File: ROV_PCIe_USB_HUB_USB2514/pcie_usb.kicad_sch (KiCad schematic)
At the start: 37 parts, among them U1 UPD720201K8-701-BAC-A, U2 SST25VF512A-33-4C-SAE, Y1 ABM8-24.000MHZ-B2-T

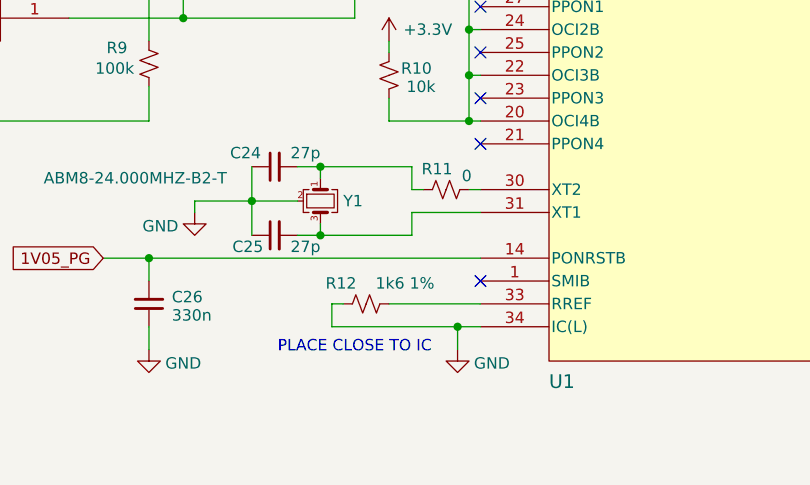
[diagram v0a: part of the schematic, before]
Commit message: updates
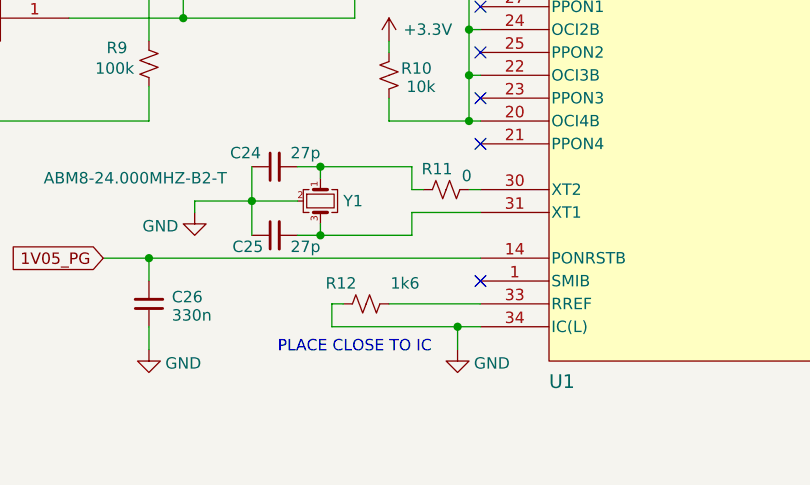
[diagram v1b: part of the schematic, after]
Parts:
- C10: Part Number CL21A106KOQNNNE -> CL21A106KOQNNNE
- C11, C12, C13, C14, C15, C16, C17, C18, C19, C20, C22, C23, C3, C4, C5, C6, C7, C8: Part Number CL05B104KB5NNNC -> CL05B104KO5NNNC
- C21, C9: footprint Capacitor_SMD:C_1206_3216Metric -> Capacitor_SMD:C_0805_2012Metric; Part Number CL31B226MPHNNNE -> CL21A226MOQNNNE
- C24, C25: Part Number CL05C270JB51PNC -> CL05C270JB5NNNC
- R10, R4, R5, R6, R7, R8: Part Number AC0603FR-0710KL -> RC0603FR-0710KL
- R11: Part Number AC0402FR-070RL -> RC0402JR-070RL
- R12: value 1k6 1% -> 1k6; Part Number RT0603BRD071K6L -> RC0603FR-071K6L
- R9: Part Number AC0603FR-07100KL -> RC0603FR-07100KL
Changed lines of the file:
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@@
 			)
 		)
-		(property "Part Number" "AC0603FR-0710KL"
+		(property "Part Number" "RC0603FR-0710KL"
 			(at 107.95 116.84 0)
 			(hide yes)
@@
 			)
 		)
-		(property "Part Number" "CL05B104KB5NNNC"
+		(property "Part Number" "CL05B104KO5NNNC"
 			(at 29.21 29.21 0)
 			(hide yes)
@@
 			)
 		)
-		(property "Part Number" "AC0603FR-07100KL"
+		(property "Part Number" "RC0603FR-07100KL"
 			(at 81.28 115.57 0)
 			(hide yes)
@@
 			)
 		)
-		(property "Part Number" "CL05B104KB5NNNC"
+		(property "Part Number" "CL05B104KO5NNNC"
 			(at 39.37 46.99 0)
 			(hide yes)
@@
 			)
 		)
-		(property "Part Number" "CL05B104KB5NNNC"
+		(property "Part Number" "CL05B104KO5NNNC"
 			(at 91.44 59.69 90)
 			(hide yes)
@@
 			)
 		)
-		(property "Part Number" "AC0402FR-070RL"
+		(property "Part Number" "RC0402JR-070RL"
 			(at 114.3 129.54 90)
 			(hide yes)
@@
 			)
 		)
-		(property "Part Number" "AC0603FR-0710KL"
+		(property "Part Number" "RC0603FR-0710KL"
 			(at 85.09 96.52 0)
 			(hide yes)
@@
 			)
 		)
-		(property "Part Number" "CL05C270JB51PNC"
+		(property "Part Number" "CL05C270JB5NNNC"
 			(at 95.25 127 90)
 			(hide yes)
@@
 			)
 		)
-		(property "Part Number" "CL05B104KB5NNNC"
+		(property "Part Number" "CL05B104KO5NNNC"
 			(at 34.29 29.21 0)
 			(hide yes)
@@
 			)
 		)
-		(property "Part Number" "CL05B104KB5NNNC"
+		(property "Part Number" "CL05B104KO5NNNC"
 			(at 64.77 46.99 0)
 			(hide yes)
@@
 			)
 		)
-		(property "Footprint" "Capacitor_SMD:C_1206_3216Metric"
+		(property "Footprint" "Capacitor_SMD:C_0805_2012Metric"
 			(at 64.77 29.21 0)
 			(hide yes)
@@
 			)
 		)
-		(property "Part Number" "CL31B226MPHNNNE"
+		(property "Part Number" "CL21A226MOQNNNE"
 			(at 64.77 29.21 0)
 			(hide yes)
@@
 			)
 		)
-		(property "Part Number" "CL05B104KB5NNNC"
+		(property "Part Number" "CL05B104KO5NNNC"
 			(at 49.53 29.21 0)
 			(hide yes)
@@
 			)
 		)
-		(property "Part Number" "CL05B104KB5NNNC"
+		(property "Part Number" "CL05B104KO5NNNC"
 			(at 34.29 46.99 0)
 			(hide yes)
@@
 			)
 		)
-		(property "Part Number" "CL05C270JB51PNC"
+		(property "Part Number" "CL05C270JB5NNNC"
 			(at 95.25 134.62 90)
 			(hide yes)
@@
 			)
 		)
-		(property "Part Number" "CL05B104KB5NNNC"
+		(property "Part Number" "CL05B104KO5NNNC"
 			(at 223.52 39.37 0)
 			(hide yes)
@@
 			)
 		)
-		(property "Part Number" "AC0603FR-0710KL"
+		(property "Part Number" "RC0603FR-0710KL"
 			(at 77.47 96.52 0)
 			(hide yes)
@@
 			)
 		)
-		(property "Footprint" "Capacitor_SMD:C_1206_3216Metric"
+		(property "Footprint" "Capacitor_SMD:C_0805_2012Metric"
 			(at 73.66 46.99 0)
 			(hide yes)
@@
 			)
 		)
-		(property "Part Number" "CL31B226MPHNNNE"
+		(property "Part Number" "CL21A226MOQNNNE"
 			(at 73.66 46.99 0)
 			(hide yes)
@@
 			)
 		)
-		(property "Part Number" "CL05B104KB5NNNC"
+		(property "Part Number" "CL05B104KO5NNNC"
 			(at 59.69 46.99 0)
 			(hide yes)
@@
 			)
 		)
-		(property "Part Number" "CL05B104KB5NNNC"
+		(property "Part Number" "CL05B104KO5NNNC"
 			(at 49.53 46.99 0)
 			(hide yes)
@@
 			)
 		)
-		(property "Part Number" "AC0603FR-0710KL"
+		(property "Part Number" "RC0603FR-0710KL"
 			(at 73.66 96.52 0)
 			(hide yes)
@@
 			)
 		)
-		(property "Part Number" "CL05B104KB5NNNC"
+		(property "Part Number" "CL05B104KO5NNNC"
 			(at 44.45 46.99 0)
 			(hide yes)
@@
 			)
 		)
-		(property "Part Number" "CL05B104KB5NNNC"
+		(property "Part Number" "CL05B104KO5NNNC"
 			(at 91.44 62.23 90)
 			(hide yes)
@@
 			)
 		)
-		(property "Part Number" "CL21A106KOQNNNE"
+		(property "Part Number" "CL21A106KOQNNNE "
 			(at 213.36 39.37 0)
 			(hide yes)
@@
 			)
 		)
-		(property "Part Number" "CL05B104KB5NNNC"
+		(property "Part Number" "CL05B104KO5NNNC"
 			(at 39.37 29.21 0)
 			(hide yes)
@@
 			)
 		)
-		(property "Part Number" "CL05B104KB5NNNC"
+		(property "Part Number" "CL05B104KO5NNNC"
 			(at 44.45 29.21 0)
 			(hide yes)
@@
 			)
 		)
-		(property "Value" "1k6 1%"
+		(property "Value" "1k6"
 			(at 109.728 139.954 90)
 			(show_name no)
@@
 			)
 		)
-		(property "Part Number" "RT0603BRD071K6L"
+		(property "Part Number" "RC0603FR-071K6L"
 			(at 105.41 142.24 90)
 			(hide yes)
@@
 			)
 		)
-		(property "Part Number" "CL05B104KB5NNNC"
+		(property "Part Number" "CL05B104KO5NNNC"
 			(at 54.61 46.99 0)
 			(hide yes)
@@
 			)
 		)
-		(property "Part Number" "CL05B104KB5NNNC"
+		(property "Part Number" "CL05B104KO5NNNC"
 			(at 54.61 29.21 0)
 			(hide yes)
@@
 			)
 		)
-		(property "Part Number" "CL05B104KB5NNNC"
+		(property "Part Number" "CL05B104KO5NNNC"
 			(at 228.6 39.37 0)
 			(hide yes)
@@
 			)
 		)
-		(property "Part Number" "AC0603FR-0710KL"
+		(property "Part Number" "RC0603FR-0710KL"
 			(at 81.28 77.47 0)
 			(hide yes)
@@
 			)
 		)
-		(property "Part Number" "AC0603FR-0710KL"
+		(property "Part Number" "RC0603FR-0710KL"
 			(at 38.1 101.6 0)
 			(hide yes)
@@
 			)
 		)
-		(property "Part Number" "CL05B104KB5NNNC"
+		(property "Part Number" "CL05B104KO5NNNC"
 			(at 29.21 46.99 0)
 			(hide yes)

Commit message: changes
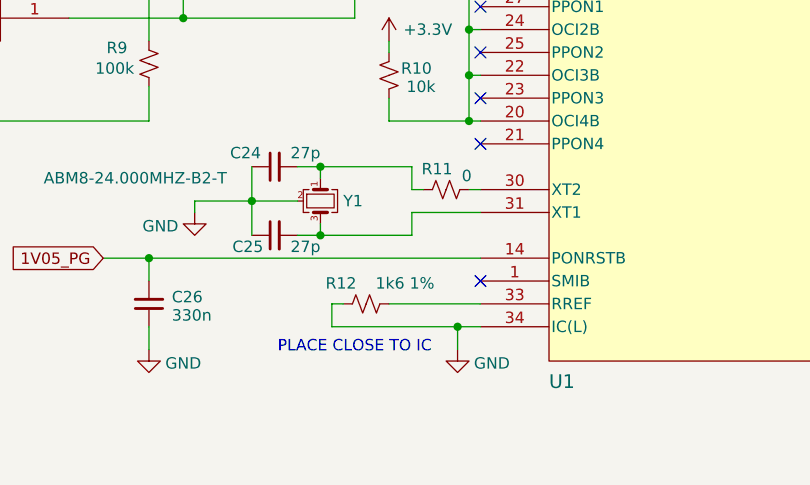
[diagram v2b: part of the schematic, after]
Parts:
- C10: Part Number CL21A106KOQNNNE -> CC0805KRX5R8BB106
- C11, C12, C13, C14, C15, C16, C17, C18, C19, C20, C22, C23, C3, C4, C5, C6, C7, C8: Part Number CL05B104KO5NNNC -> CC0402KRX7R8BB104
- C21, C9: footprint Capacitor_SMD:C_0805_2012Metric -> Capacitor_SMD:C_1206_3216Metric; Part Number CL21A226MOQNNNE -> CC1206KKX5R8BB226
- C24, C25: Part Number CL05C270JB5NNNC -> CC0402JRNPO9BN270
- C26: Part Number CL05A334KQ5NNNC -> CC0402KPX5R6BB334
- R12: value 1k6 -> 1k6 1%
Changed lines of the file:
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@@
 			)
 		)
-		(property "Part Number" "CL05B104KO5NNNC"
+		(property "Part Number" "CC0402KRX7R8BB104"
 			(at 29.21 29.21 0)
 			(hide yes)
@@
 			)
 		)
-		(property "Part Number" "CL05B104KO5NNNC"
+		(property "Part Number" "CC0402KRX7R8BB104"
 			(at 39.37 46.99 0)
 			(hide yes)
@@
 			)
 		)
-		(property "Part Number" "CL05B104KO5NNNC"
+		(property "Part Number" "CC0402KRX7R8BB104"
 			(at 91.44 59.69 90)
 			(hide yes)
@@
 			)
 		)
-		(property "Part Number" "CL05C270JB5NNNC"
+		(property "Part Number" "CC0402JRNPO9BN270"
 			(at 95.25 127 90)
 			(hide yes)
@@
 			)
 		)
-		(property "Part Number" "CL05B104KO5NNNC"
+		(property "Part Number" "CC0402KRX7R8BB104"
 			(at 34.29 29.21 0)
 			(hide yes)
@@
 			)
 		)
-		(property "Part Number" "CL05B104KO5NNNC"
+		(property "Part Number" "CC0402KRX7R8BB104"
 			(at 64.77 46.99 0)
 			(hide yes)
@@
 			)
 		)
-		(property "Footprint" "Capacitor_SMD:C_0805_2012Metric"
+		(property "Footprint" "Capacitor_SMD:C_1206_3216Metric"
 			(at 64.77 29.21 0)
 			(hide yes)
@@
 			)
 		)
-		(property "Part Number" "CL21A226MOQNNNE"
+		(property "Part Number" "CC1206KKX5R8BB226"
 			(at 64.77 29.21 0)
 			(hide yes)
@@
 			)
 		)
-		(property "Part Number" "CL05B104KO5NNNC"
+		(property "Part Number" "CC0402KRX7R8BB104"
 			(at 49.53 29.21 0)
 			(hide yes)
@@
 			)
 		)
-		(property "Part Number" "CL05B104KO5NNNC"
+		(property "Part Number" "CC0402KRX7R8BB104"
 			(at 34.29 46.99 0)
 			(hide yes)
@@
 			)
 		)
-		(property "Part Number" "CL05C270JB5NNNC"
+		(property "Part Number" "CC0402JRNPO9BN270"
 			(at 95.25 134.62 90)
 			(hide yes)
@@
 			)
 		)
-		(property "Part Number" "CL05B104KO5NNNC"
+		(property "Part Number" "CC0402KRX7R8BB104"
 			(at 223.52 39.37 0)
 			(hide yes)
@@
 			)
 		)
-		(property "Footprint" "Capacitor_SMD:C_0805_2012Metric"
+		(property "Footprint" "Capacitor_SMD:C_1206_3216Metric"
 			(at 73.66 46.99 0)
 			(hide yes)
@@
 			)
 		)
-		(property "Part Number" "CL21A226MOQNNNE"
+		(property "Part Number" "CC1206KKX5R8BB226"
 			(at 73.66 46.99 0)
 			(hide yes)
@@
 			)
 		)
-		(property "Part Number" "CL05B104KO5NNNC"
+		(property "Part Number" "CC0402KRX7R8BB104"
 			(at 59.69 46.99 0)
 			(hide yes)
@@
 			)
 		)
-		(property "Part Number" "CL05B104KO5NNNC"
+		(property "Part Number" "CC0402KRX7R8BB104"
 			(at 49.53 46.99 0)
 			(hide yes)
@@
 			)
 		)
-		(property "Part Number" "CL05B104KO5NNNC"
+		(property "Part Number" "CC0402KRX7R8BB104"
 			(at 44.45 46.99 0)
 			(hide yes)
@@
 			)
 		)
-		(property "Part Number" "CL05B104KO5NNNC"
+		(property "Part Number" "CC0402KRX7R8BB104"
 			(at 91.44 62.23 90)
 			(hide yes)
@@
 			)
 		)
-		(property "Part Number" "CL21A106KOQNNNE "
+		(property "Part Number" "CC0805KRX5R8BB106"
 			(at 213.36 39.37 0)
 			(hide yes)
@@
 			)
 		)
-		(property "Part Number" "CL05B104KO5NNNC"
+		(property "Part Number" "CC0402KRX7R8BB104"
 			(at 39.37 29.21 0)
 			(hide yes)
@@
 			)
 		)
-		(property "Part Number" "CL05B104KO5NNNC"
+		(property "Part Number" "CC0402KRX7R8BB104"
 			(at 44.45 29.21 0)
 			(hide yes)
@@
 			)
 		)
-		(property "Value" "1k6"
+		(property "Value" "1k6 1%"
 			(at 109.728 139.954 90)
 			(show_name no)
@@
 			)
 		)
-		(property "Part Number" "CL05B104KO5NNNC"
+		(property "Part Number" "CC0402KRX7R8BB104"
 			(at 54.61 46.99 0)
 			(hide yes)
@@
 			)
 		)
-		(property "Part Number" "CL05B104KO5NNNC"
+		(property "Part Number" "CC0402KRX7R8BB104"
 			(at 54.61 29.21 0)
 			(hide yes)
@@
 			)
 		)
-		(property "Part Number" "CL05B104KO5NNNC"
+		(property "Part Number" "CC0402KRX7R8BB104"
 			(at 228.6 39.37 0)
 			(hide yes)
@@
 			)
 		)
-		(property "Part Number" "CL05B104KO5NNNC"
+		(property "Part Number" "CC0402KRX7R8BB104"
 			(at 29.21 46.99 0)
 			(hide yes)
@@
 			)
 		)
-		(property "Part Number" "CL05A334KQ5NNNC"
+		(property "Part Number" "CC0402KPX5R6BB334"
 			(at 81.28 142.24 0)
 			(hide yes)
